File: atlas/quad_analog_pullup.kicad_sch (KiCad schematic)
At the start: 29 parts, among them U1101 MCP6004, U1102 SRV05-4, U1103 NC7SB3157P6X, U1104 NC7SB3157P6X

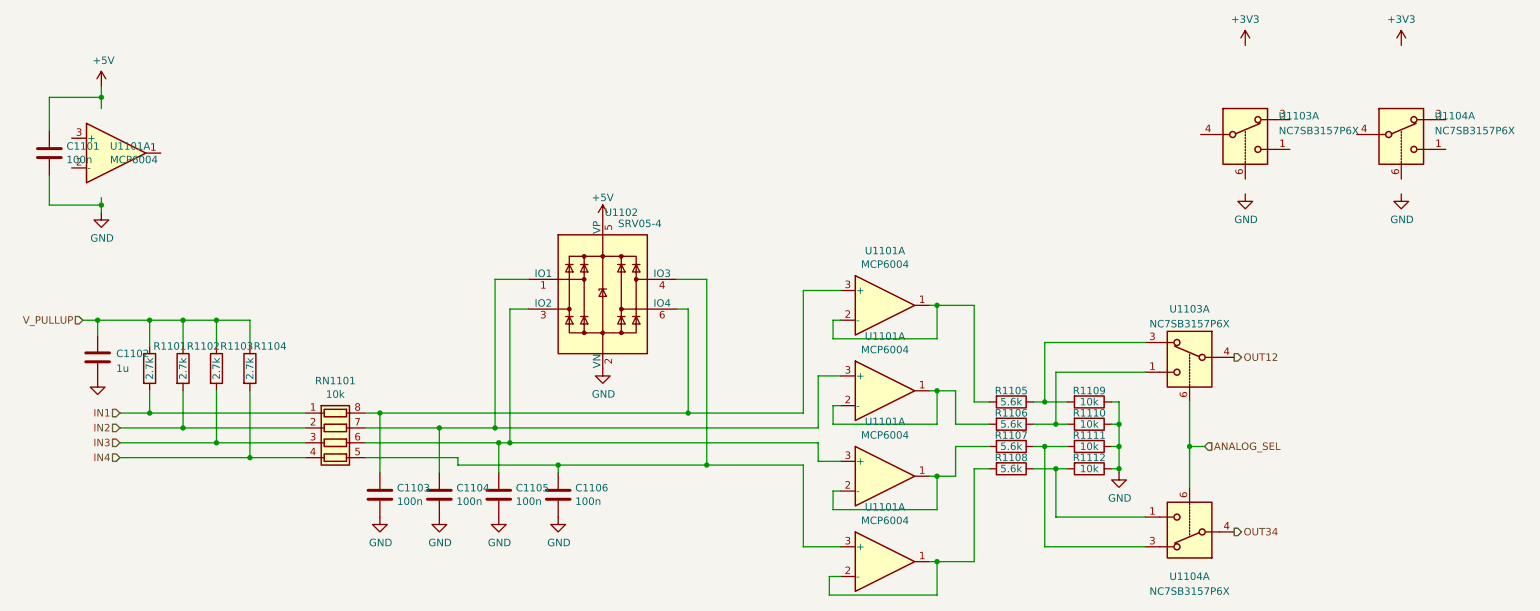
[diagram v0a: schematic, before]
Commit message: progressssss
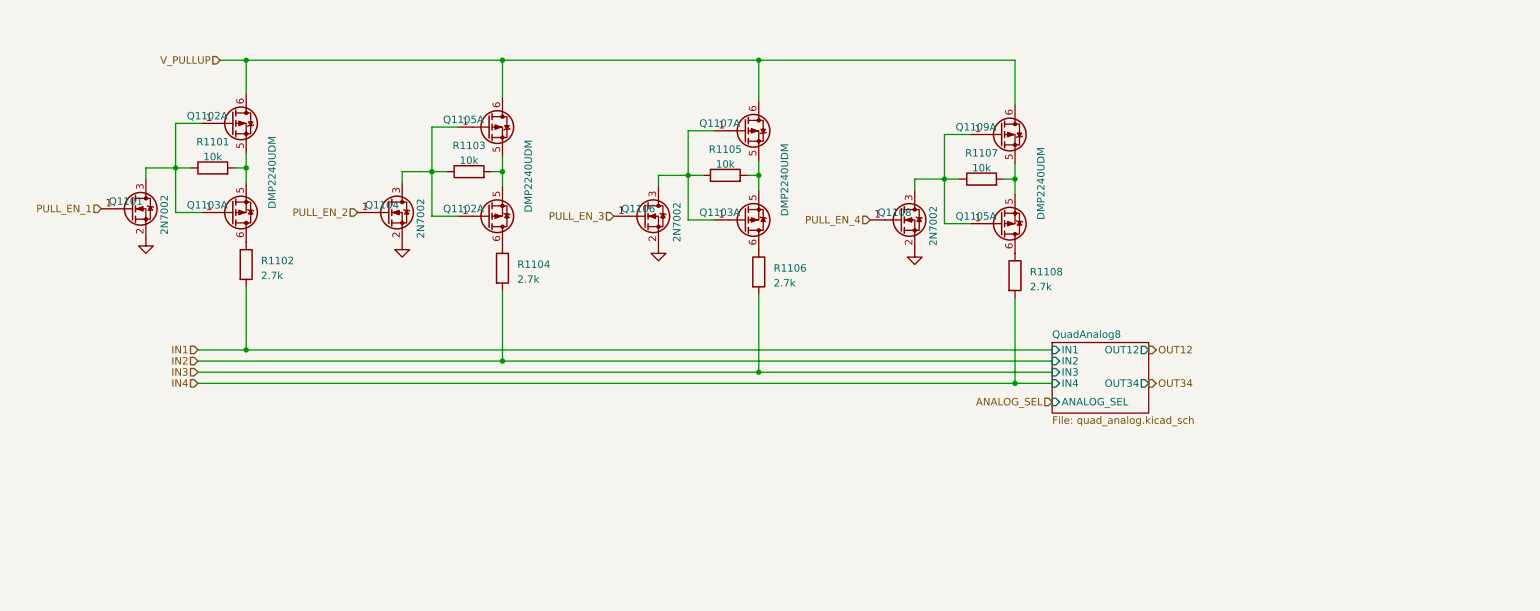
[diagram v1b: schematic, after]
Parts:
- removed C1101: 100n, Capacitor_SMD:C_0603_1608Metric, symbol Device:C
- removed C1102: 1u, symbol Device:C
- removed C1103, C1104, C1105, C1106: 100n, Capacitor_SMD:C_0402_1005Metric, symbol Device:C
- removed R1109, R1110, R1111, R1112: 10k, Resistor_SMD:R_0402_1005Metric, symbol Device:R
- removed RN1101: 10k, Resistor_SMD:R_Array_Convex_4x0603, symbol Device:R_Pack04
- removed U1101 (x5): MCP6004, Package_SO:TSSOP-14_4.4x5mm_P0.65mm, symbol Amplifier_Operational:MCP6004
- removed U1102: SRV05-4, Package_TO_SOT_SMD:SOT-23-6, symbol Power_Protection:SRV05-4
- removed U1103 (x2), U1104 (x2): NC7SB3157P6X, Package_TO_SOT_SMD:SOT-363_SC-70-6, symbol Analog_Switch:NC7SB3157P6X
- added Q1101, Q1104, Q1106, Q1108: 2N7002, Package_TO_SOT_SMD:SOT-23, symbol Device:Q_NMOS_GSD
- added Q1102 (x2), Q1103 (x2), Q1105 (x2), Q1107, Q1109: DMP2240UDM, Package_TO_SOT_SMD:SOT-23-6, symbol Device:Q_Dual_PMOS_G1S2G2D2S1D1
- R1101, R1103: value 2.7k -> 10k; footprint (none) -> Resistor_SMD:R_0603_1608Metric; LCSC (none) -> C25804
- R1102, R1104: footprint (none) -> Resistor_SMD:R_0603_1608Metric; LCSC (none) -> C13167
- R1105, R1107: value 5.6k -> 10k; footprint Resistor_SMD:R_0402_1005Metric -> Resistor_SMD:R_0603_1608Metric; LCSC C25908 -> C25804
- R1106, R1108: value 5.6k -> 2.7k; footprint Resistor_SMD:R_0402_1005Metric -> Resistor_SMD:R_0603_1608Metric; LCSC C25908 -> C13167
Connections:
- net GND: now also Q1101.2 (S), Q1104.2 (S), Q1106.2 (S), Q1108.2 (S)
- net IN1: now also R1102.2; no longer R1101.2
- net IN2: now also R1104.2; no longer R1102.2
- net IN3: now also R1106.2; no longer R1103.2
- net IN4: now also R1108.2; no longer R1104.2
- net V_PULLUP: now also Q1102.6 (D), Q1105.6 (D), Q1107.6 (D), Q1109.6 (D); no longer R1101.1, R1102.1, R1103.1, R1104.1
- net at R1106.1: now also Q1103.6 (D)
- net at R1107.1: now also Q1105.1 (G), Q1108.3 (D), Q1109.1 (G)
- net at R1108.1: now also Q1105.6 (D)
- net at R1107.2: now also Q1105.5 (S), Q1109.5 (S)
- net at R1105.1: now also Q1103.1 (G), Q1106.3 (D), Q1107.1 (G)
- net at R1105.2: now also Q1103.5 (S), Q1107.5 (S)
- new net: Q1101.3 (D), Q1102.1 (G), Q1103.1 (G), R1101.1
- new net: Q1102.5 (S), Q1103.5 (S), R1101.2
- new net: Q1102.6 (D), R1104.1
- new net: Q1102.1 (G), Q1104.3 (D), Q1105.1 (G), R1103.1
- new net: Q1102.5 (S), Q1105.5 (S), R1103.2
- new net: Q1103.6 (D), R1102.1
- new net PULL_EN_1: Q1101.1 (G)
- new net PULL_EN_2: Q1104.1 (G)
- new net PULL_EN_3: Q1106.1 (G)
- new net PULL_EN_4: Q1108.1 (G)
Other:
- added sheet QuadAnalog8 (quad_analog.kicad_sch)

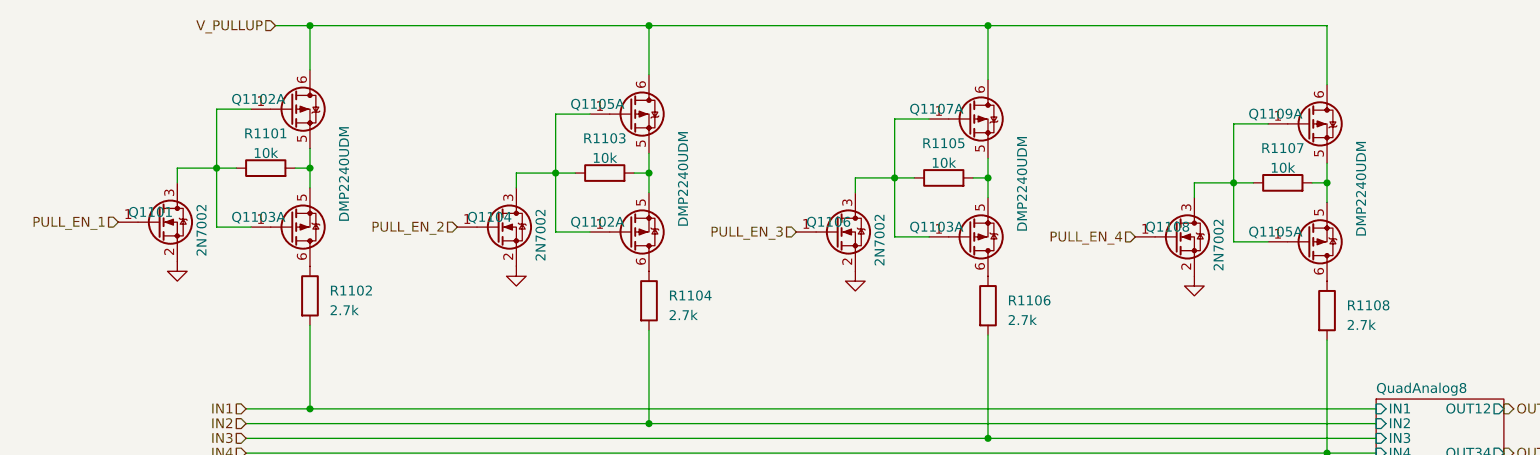
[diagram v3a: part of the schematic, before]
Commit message: upgrade kicad
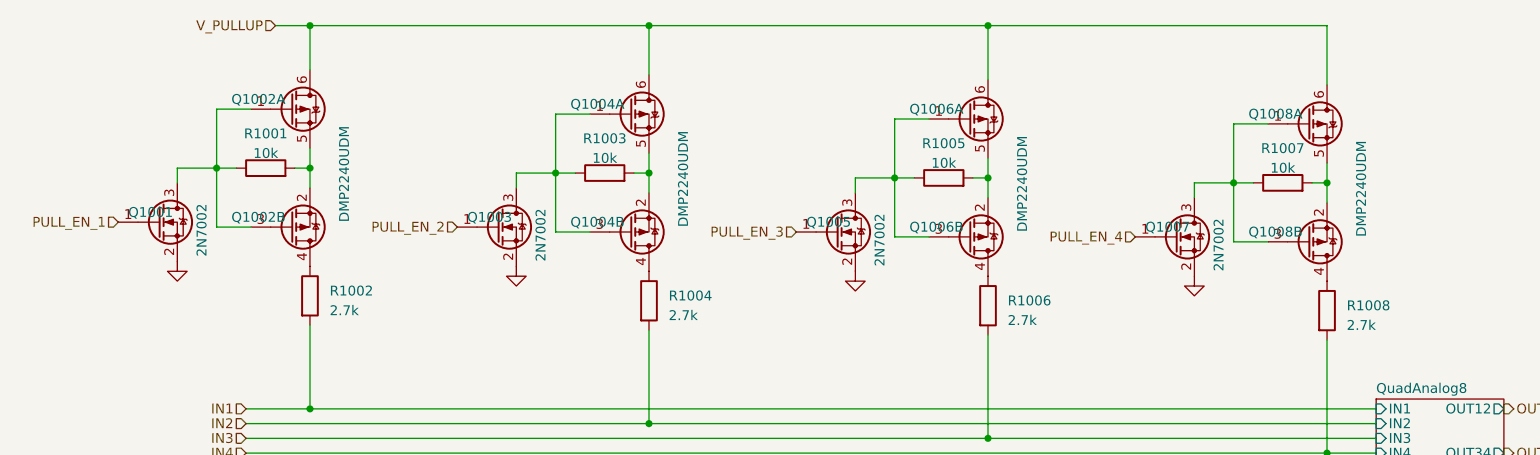
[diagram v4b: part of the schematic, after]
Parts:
- renumbered Q1101 to Q1001, Q1102 to Q1002, Q1103 to Q1002, Q1104 to Q1003, Q1105 to Q1004, Q1102 to Q1004, Q1106 to Q1005, Q1107 to Q1006, Q1103 to Q1006, Q1108 to Q1007, Q1105 to Q1008, Q1109 to Q1008, R1101 to R1001, R1102 to R1002, R1103 to R1003, R1104 to R1004, R1105 to R1005, R1106 to R1006, R1107 to R1007, R1108 to R1008
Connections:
- net at Q1007.3 (D), Q1008.1 (G), R1007.1: now also Q1008.3 (G); no longer Q1008.1 (G)
- net at Q1008.5 (S), R1007.2: now also Q1008.2 (S); no longer Q1008.5 (S)
- net at R1008.1: now also Q1008.4 (D); no longer Q1008.6 (D)
- net at Q1005.3 (D), Q1006.1 (G), R1005.1: now also Q1006.3 (G); no longer Q1006.1 (G)
- net at Q1006.5 (S), R1005.2: now also Q1006.2 (S); no longer Q1006.5 (S)
- net at R1006.1: now also Q1006.4 (D); no longer Q1006.6 (D)
- net at Q1001.3 (D), Q1002.1 (G), R1001.1: now also Q1002.3 (G); no longer Q1002.1 (G)
- net at Q1002.5 (S), R1001.2: now also Q1002.2 (S); no longer Q1002.5 (S)
- net at R1004.1: now also Q1004.4 (D); no longer Q1004.6 (D)
- net at Q1003.3 (D), Q1004.1 (G), R1003.1: now also Q1004.3 (G); no longer Q1004.1 (G)
- net at Q1004.5 (S), R1003.2: now also Q1004.2 (S); no longer Q1004.5 (S)
- net at R1002.1: now also Q1002.4 (D); no longer Q1002.6 (D)
